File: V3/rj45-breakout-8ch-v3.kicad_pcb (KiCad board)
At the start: 2 copper layers, 93 x 67.8 mm, 14 parts, among them J1 Jack RJ45, J10 SWITCHES1, J11 SWITCHES2, J12 SWITCHES3, J13 SWITCHES4, J2 Jack RJ45, J3 Jack RJ45, J4 Jack RJ45, J5 Jack RJ45, J6 Jack RJ45, J7 Jack RJ45, J8 Jack RJ45, J9 24V

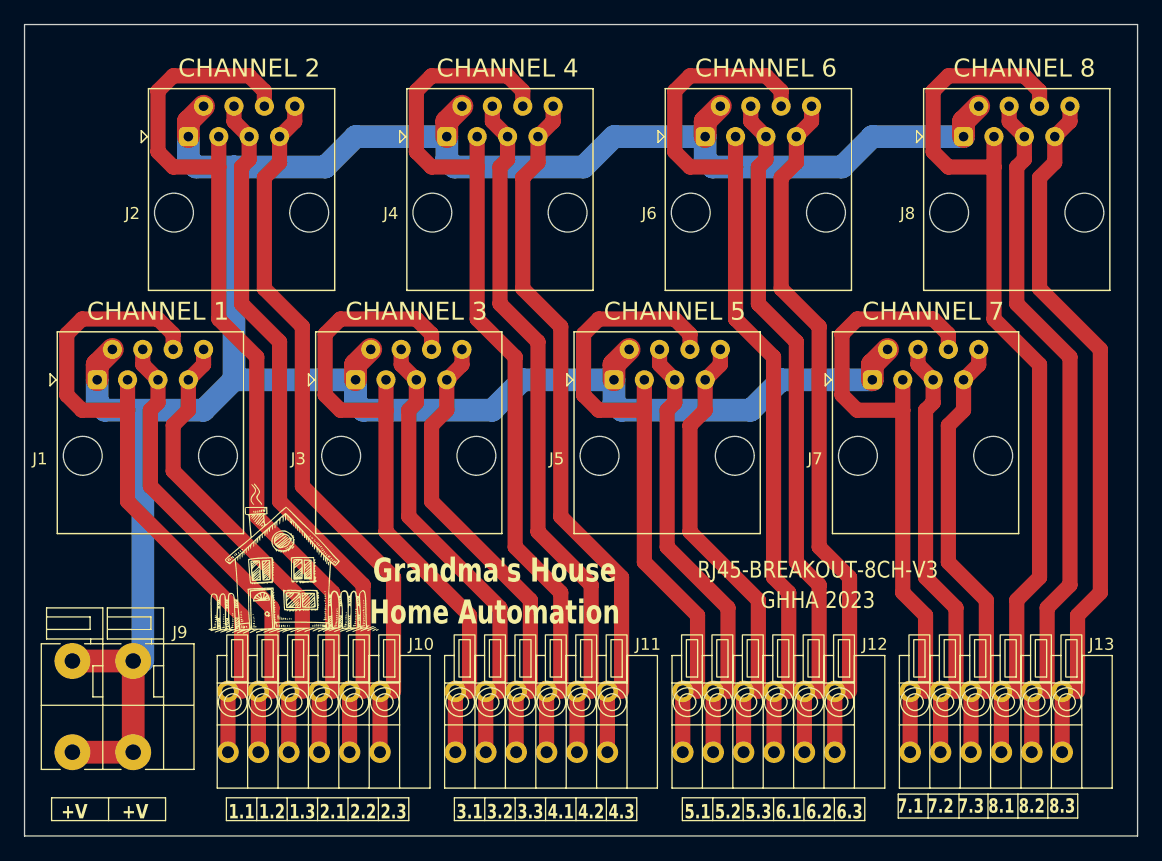
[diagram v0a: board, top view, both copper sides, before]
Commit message: Update rj45-breakout-8ch-v3.kicad_pcb
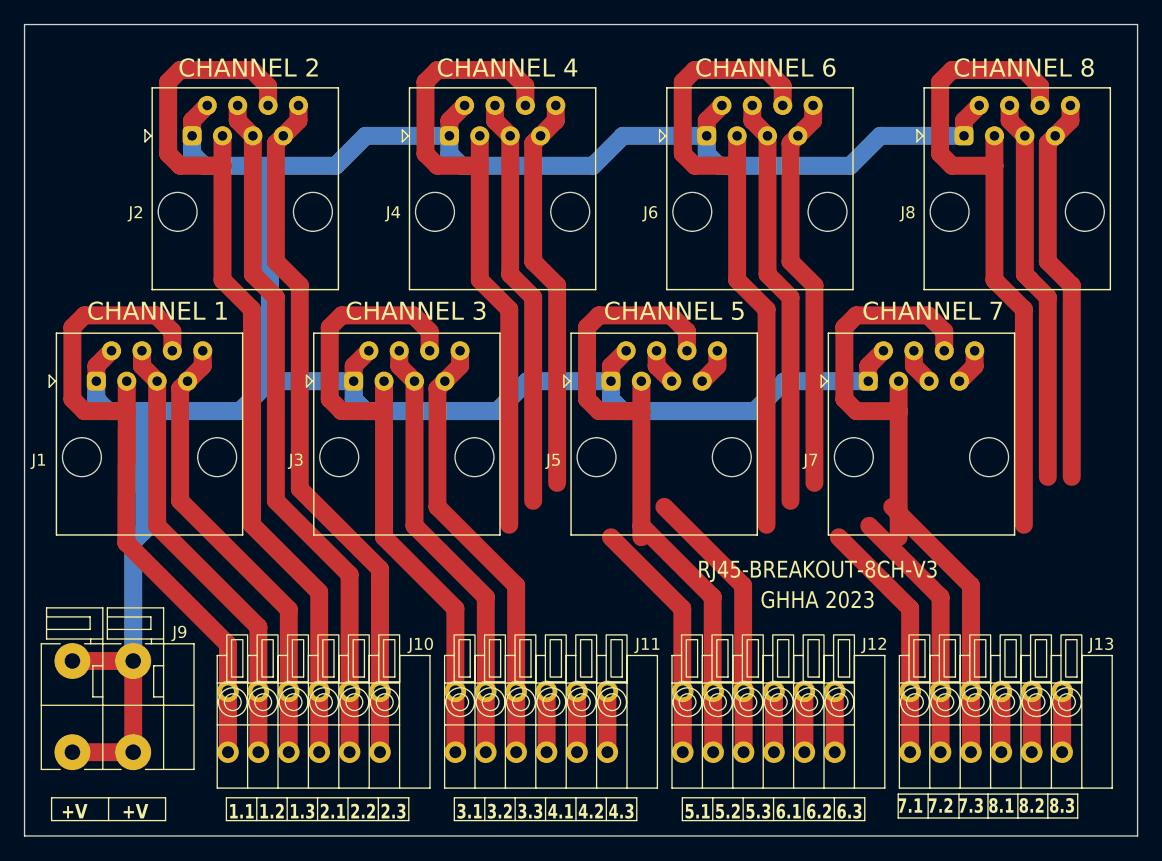
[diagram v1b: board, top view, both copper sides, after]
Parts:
- removed ?: , Tales:Grandmas_medium
- moved J7 0.36 mm to (174.9, 92.0)
- moved J2 0.32 mm to (118.4, 71.5)
- moved J5 0.28 mm to (153.4, 92.0)
- moved J4 0.23 mm to (139.9, 71.5)
- moved J3 0.20 mm to (131.9, 92.0)
- moved J6 0.15 mm to (161.4, 71.5)
- moved J1 0.13 mm to (110.4, 92.0)
- moved J8 0.08 mm to (182.9, 71.5)
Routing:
- net Net-(J12-Pin_2): track 36.5 -> 8.15 mm
- net Net-(J13-Pin_3): track 36.0 -> 8.15 mm
- net Net-(J13-Pin_2): track 35.5 -> 8.15 mm
- net Net-(J11-Pin_6): track 58.4 -> 38.2 mm
- net Net-(J13-Pin_6): track 57.9 -> 37.7 mm
- net Net-(J12-Pin_6): track 57.4 -> 38.2 mm
- net Net-(J11-Pin_5): track 57.9 -> 39.4 mm
- net Net-(J12-Pin_5): track 56.9 -> 39.4 mm
- net Net-(J11-Pin_4): track 76.2 -> 60.5 mm
- net Net-(J12-Pin_4): track 75.2 -> 60.5 mm
- net Net-(J12-Pin_3): track 37.1 -> 42.6 mm
- net Net-(J13-Pin_5): track 57.4 -> 55.6 mm
- net Net-(J9-Pin_1): track 229.9 -> 228.3 mm
- net Net-(J13-Pin_1): track 53.8 -> 55.4 mm
- net Net-(J13-Pin_4): track 75.7 -> 76.8 mm
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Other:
- board text removed: "Grandma's House"
- board text removed: "Home Automation"
